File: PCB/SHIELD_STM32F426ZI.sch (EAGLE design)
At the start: 16 parts, among them IC1 AS4C16M16SA-6TCN, J1 104239-1430

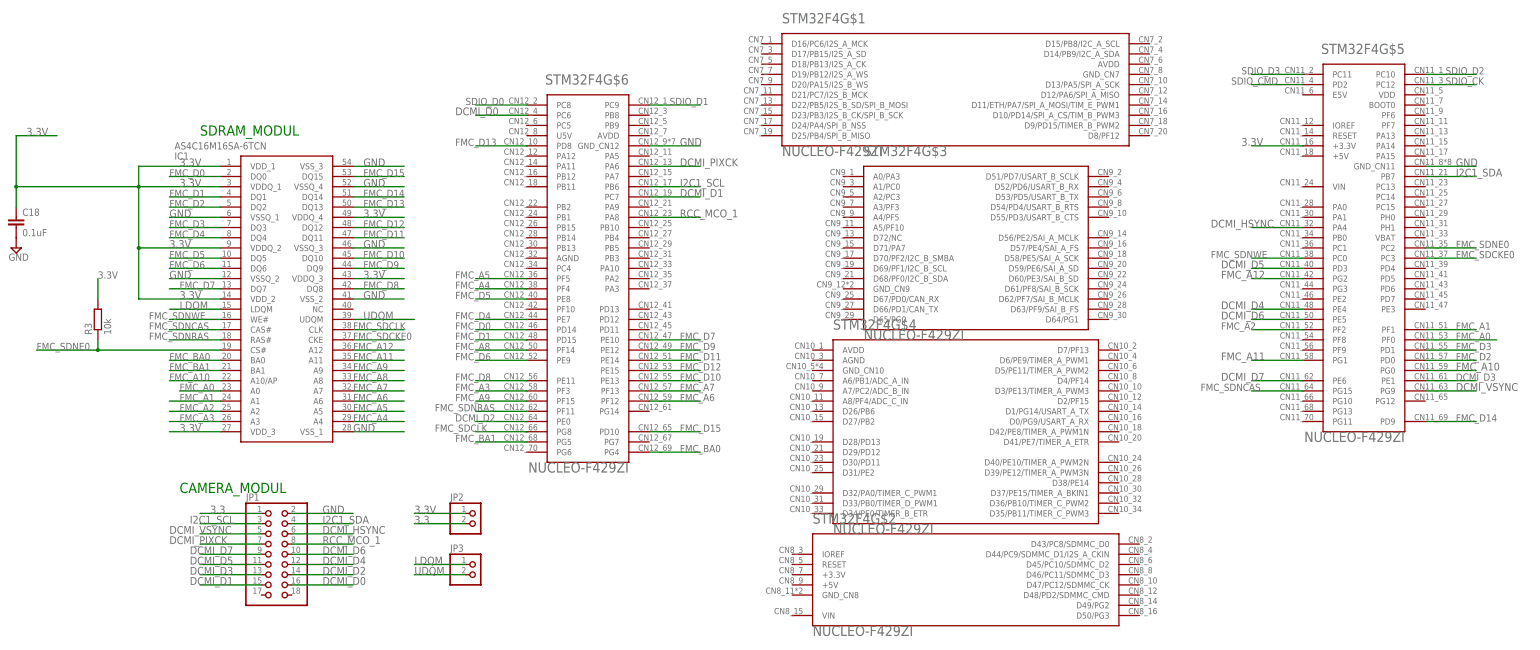
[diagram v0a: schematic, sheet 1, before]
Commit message: PCB wurde mit kurzer Leitung korrigiert
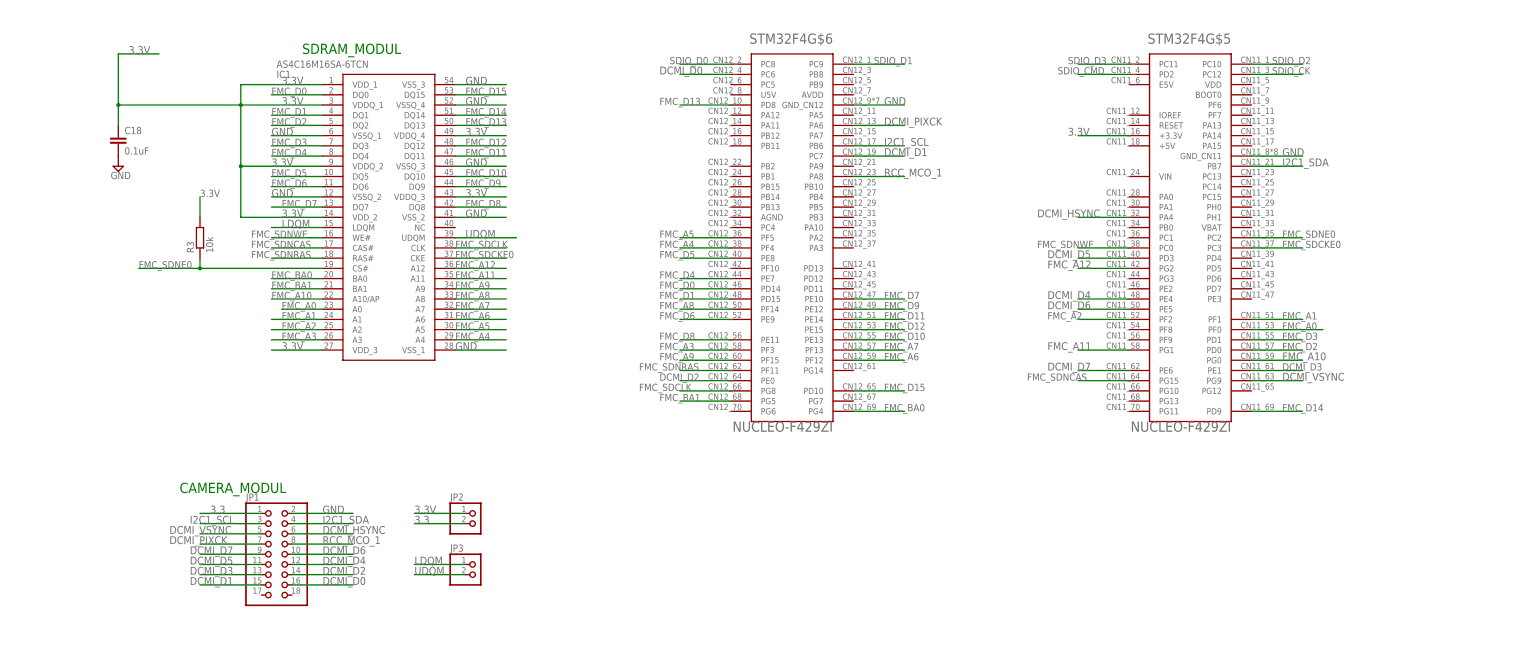
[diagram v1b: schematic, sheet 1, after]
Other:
- moved on the sheet: C18, IC1, R3, STM32F4G$5, STM32F4G$6
